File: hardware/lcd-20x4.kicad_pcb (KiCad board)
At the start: 2 copper layers, 98 x 60 mm, 30 parts, among them P1 CON-SENSOR, P2 BTN-HEADER, Q1 2N7002, SW1 SW_PUSH, SW2 SW_PUSH, SW3 SW_PUSH, SW4 SW_PUSH, U1 M24C64, U2 MCP23017, U3 PCA9306D, U4 LCD-20X4, U5 DRILL, U6 DRILL, U7 DRILL, U8 DRILL

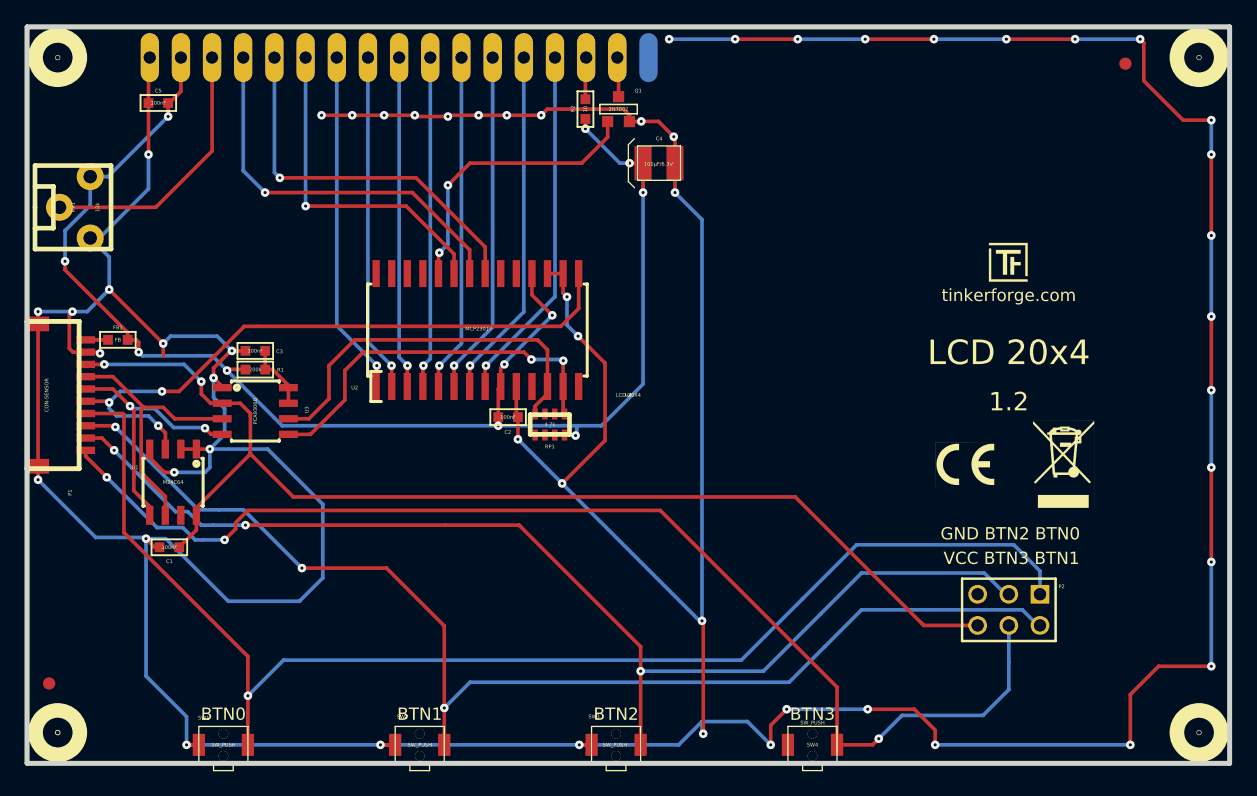
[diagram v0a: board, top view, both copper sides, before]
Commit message: Add 3d information (final)
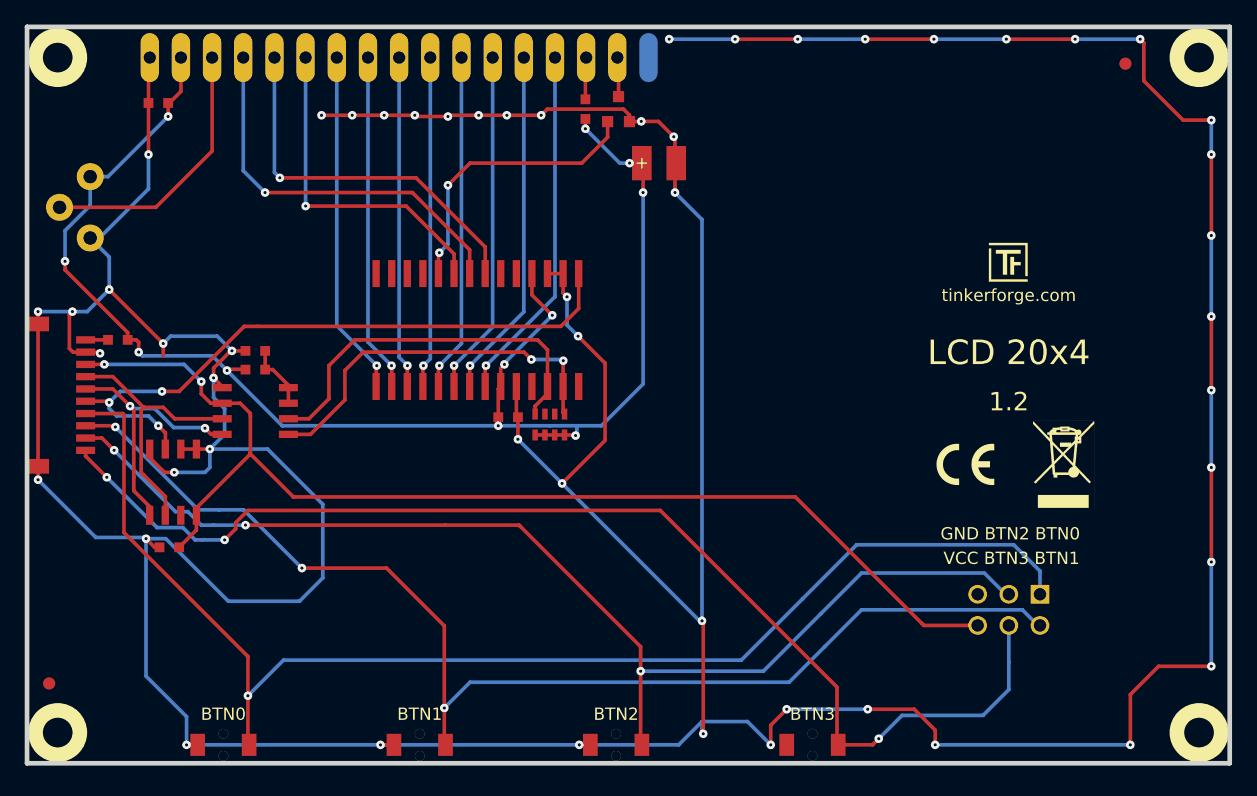
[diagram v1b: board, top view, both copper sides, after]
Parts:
- C1, C2, C3, C5, FB1: footprint 0603 -> kicad-libraries:C0603
- C4: footprint 3528-21 -> kicad-libraries:3528-21
- Fiducial_Mark (x2): footprint Fiducial_Mark -> kicad-libraries:Fiducial_Mark
- P1: footprint CON-SENSOR -> kicad-libraries:CON-SENSOR
- P2: footprint pin_array_3x2 -> kicad-libraries:pin_array_3x2
- Q1: footprint SOT23GDS -> kicad-libraries:SOT23GDS
- R1, R2: footprint 0603 -> kicad-libraries:R0603
- RP1: footprint 0603X4 -> kicad-libraries:0603X4
- RV1: footprint POT_36W -> kicad-libraries:POT_36W
- Ref**: footprint Logo_31x31 -> kicad-libraries:Logo_31x31
- SW1, SW2, SW3, SW4: footprint TACT-SWITCH -> kicad-libraries:TACT-SWITCH
- U1, U3: footprint SOIC8 -> kicad-libraries:SOIC8
- U2: footprint SOIC28 -> kicad-libraries:SOIC28
- U4: footprint LCD-20x4 -> kicad-libraries:LCD-20x4
- U5, U6, U7, U8: footprint DRILL_NP -> kicad-libraries:DRILL_NP
- VAL: footprint CE_5mm -> kicad-libraries:CE_5mm
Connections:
- RP1 pad 6: (no net) -> Net-(RP1-Pad6)
- RP1 pad 7: (no net) -> Net-(RP1-Pad7)
- U1 pad 7: (no net) -> Net-(U1-Pad7)
- U2 pad 11: (no net) -> Net-(U2-Pad11)
- U2 pad 14: (no net) -> Net-(U2-Pad14)
- U2 pad 19: (no net) -> Net-(U2-Pad19)
- U2 pad 20: (no net) -> Net-(U2-Pad20)
- U2 pad 25: (no net) -> Net-(U2-Pad25)
- U2 pad 26: (no net) -> Net-(U2-Pad26)
- U2 pad 27: (no net) -> Net-(U2-Pad27)
- U2 pad 28: (no net) -> Net-(U2-Pad28)
